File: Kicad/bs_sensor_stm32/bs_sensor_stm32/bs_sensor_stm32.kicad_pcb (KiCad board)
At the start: 2 copper layers, 1 part, among them U1 NRF24L01_Breakout

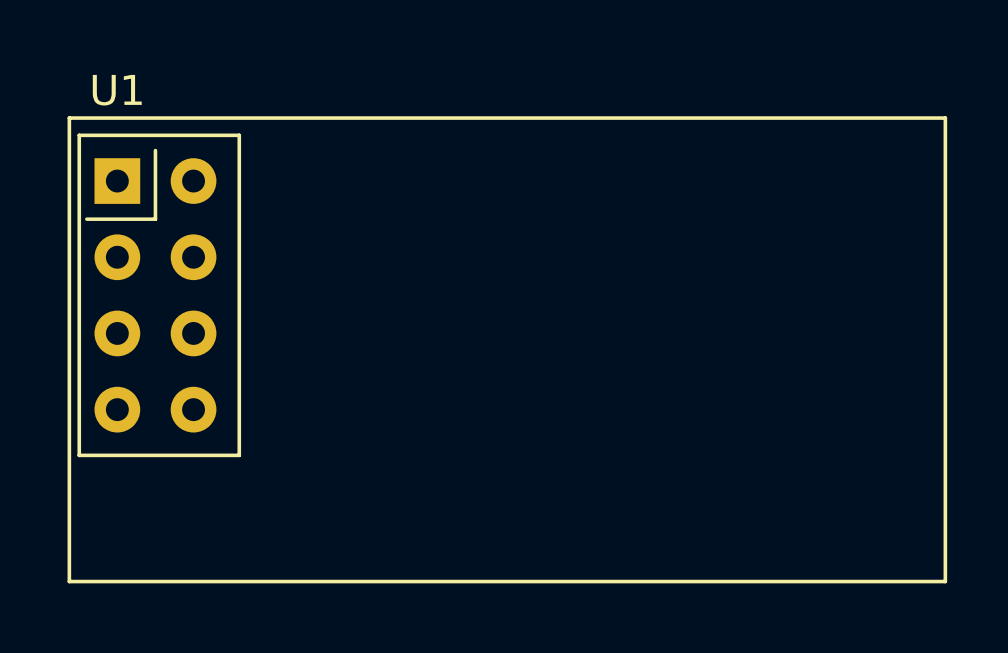
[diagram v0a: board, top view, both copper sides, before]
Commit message: 01.03.2022
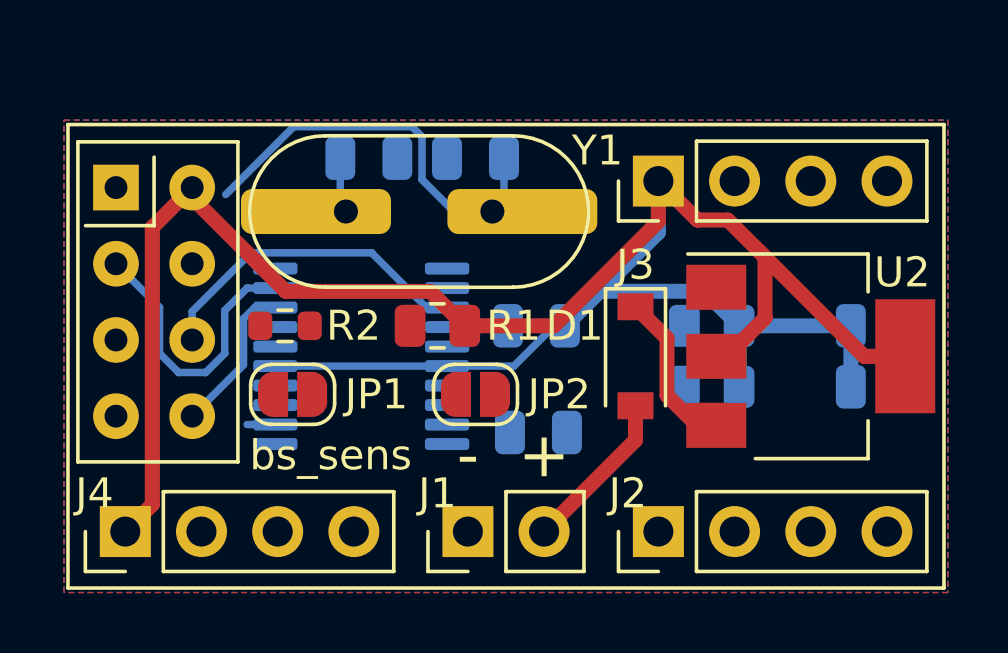
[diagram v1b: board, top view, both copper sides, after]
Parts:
- added C1: 22p, Capacitor_SMD:C_0805_2012Metric, B.Cu at (160.8, 100.8)
- added C2: 100n, Capacitor_SMD:C_0805_2012Metric, B.Cu at (177.8, 106.4)
- added C3: 10u, Capacitor_SMD:C_0805_2012Metric, B.Cu at (177.8, 108.5)
- added C4: 22p, Capacitor_SMD:C_0805_2012Metric, B.Cu at (164.3, 100.8)
- added C5: 100n, Capacitor_SMD:C_0805_2012Metric, B.Cu at (166.4, 106.4)
- added C6: 100n, Capacitor_SMD:C_0805_2012Metric, B.Cu at (166.4, 110.0)
- added D1: 1N4148W, Diode_SMD:D_SOD-123, F.Cu at (169.7, 107.4)
- added J1: Conn_01x02, Connector_PinHeader_2.54mm:PinHeader_1x02_P2.54mm_Vertical, F.Cu at (164.1, 113.3)
- added J2: Conn_01x04, Connector_PinHeader_2.54mm:PinHeader_1x04_P2.54mm_Vertical, F.Cu at (170.4, 113.3)
- added J3: Conn_01x04, Connector_PinHeader_2.54mm:PinHeader_1x04_P2.54mm_Vertical, F.Cu at (170.4, 101.6)
- added J4: Conn_01x04, Connector_PinHeader_2.54mm:PinHeader_1x04_P2.54mm_Vertical, F.Cu at (152.7, 113.3)
- added JP1: SolderJumper_2_Open, Jumper:SolderJumper-2_P1.3mm_Open_RoundedPad1.0x1.5mm, F.Cu at (158.2, 108.7)
- added JP2: SolderJumper_2_Open, Jumper:SolderJumper-2_P1.3mm_Open_RoundedPad1.0x1.5mm, F.Cu at (164.3, 108.7)
- added R1: 10k, Resistor_SMD:R_0805_2012Metric, F.Cu at (163.1, 106.4)
- added R2: 620, Resistor_SMD:R_0603_1608Metric, F.Cu at (158.0, 106.4)
- added R3: 10k, Resistor_SMD:R_0805_2012Metric, B.Cu at (172.2, 106.4)
- added R4: 4,7k, Resistor_SMD:R_0805_2012Metric, B.Cu at (172.2, 108.5)
- added U2: AMS1117-3.3, Package_TO_SOT_SMD:SOT-223-3_TabPin2, F.Cu at (175.5, 107.4)
- added U3: STM32F030F4Px, Package_SO:TSSOP-20_4.4x6.5mm_P0.65mm, B.Cu at (160.5, 107.4)
- added Y1: 16MHz, Crystal:Crystal_HC49-U_Vertical, F.Cu at (160.0, 102.6)
- moved U1 0.22 mm to (152.4, 101.8)
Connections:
- U1 pad 1: unconnected-(U1-Pad1) -> GND
- U1 pad 2: unconnected-(U1-Pad2) -> +3V3
- U1 pad 3: unconnected-(U1-Pad3) -> Net-(U1-Pad3)
- U1 pad 4: unconnected-(U1-Pad4) -> Net-(U1-Pad4)
- U1 pad 5: unconnected-(U1-Pad5) -> Net-(U1-Pad5)
- U1 pad 6: unconnected-(U1-Pad6) -> Net-(U1-Pad6)
- U1 pad 7: unconnected-(U1-Pad7) -> Net-(U1-Pad7)
- U1 pad 8: unconnected-(U1-Pad8) -> Net-(U1-Pad8)
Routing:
- net +3V3: track 0.00 -> 79.4 mm
- net Net-(C4-Pad1): track 0.00 -> 14.5 mm
- net Net-(U1-Pad6): track 0.00 -> 11.0 mm
- net Net-(U1-Pad3): track 0.00 -> 9.72 mm
- net Net-(D1-Pad2): track 0.00 -> 5.45 mm
- net Net-(D1-Pad1): track 0.00 -> 5.44 mm
- net Net-(U1-Pad8): track 0.00 -> 5.17 mm
- net Net-(C1-Pad2): track 0.00 -> 4.59 mm
- added copper zone on B.Cu, net GND
- added copper zone on F.Cu, net GND
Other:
- board text added: "+"
- board text added: "-"
- board text added: "a0"
- board text added: "a1"
- board text added: "a10"
- board text added: "a9"
- board text added: "b1"
- board text added: "bs_sens"
- board text added: "clk"
- board text added: "dio"
- board text added: "gnd"
- board text added: "nrf24l01+"
- board text added: "vcc"
